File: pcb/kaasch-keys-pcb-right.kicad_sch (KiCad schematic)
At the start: 79 parts, among them SW1 SW_Push, SW10 SW_Push, SW11 SW_Push, SW12 SW_Push, SW13 SW_Push, SW14 SW_Push, SW15 SW_Push, SW16 SW_Push, SW17 SW_Push, SW18 SW_Push, SW19 SW_Push, SW2 SW_Push, SW20 SW_Push, SW21 SW_Push, SW22 SW_Push, SW23 SW_Push, SW24 SW_Push, SW25 SW_Push, SW26 SW_Push, SW27 SW_Push, SW28 SW_Push, SW29 SW_Push, SW3 SW_Push, SW30 SW_Push, SW31 SW_Push, SW32 SW_Push, SW33 SW_Push, SW34 SW_Push, SW35 SW_Push, SW36 SW_Push_Reset, SW4 SW_Push, SW5 SW_Push, SW6 SW_Push, SW7 SW_Push, SW8 SW_Push, SW9 SW_Push

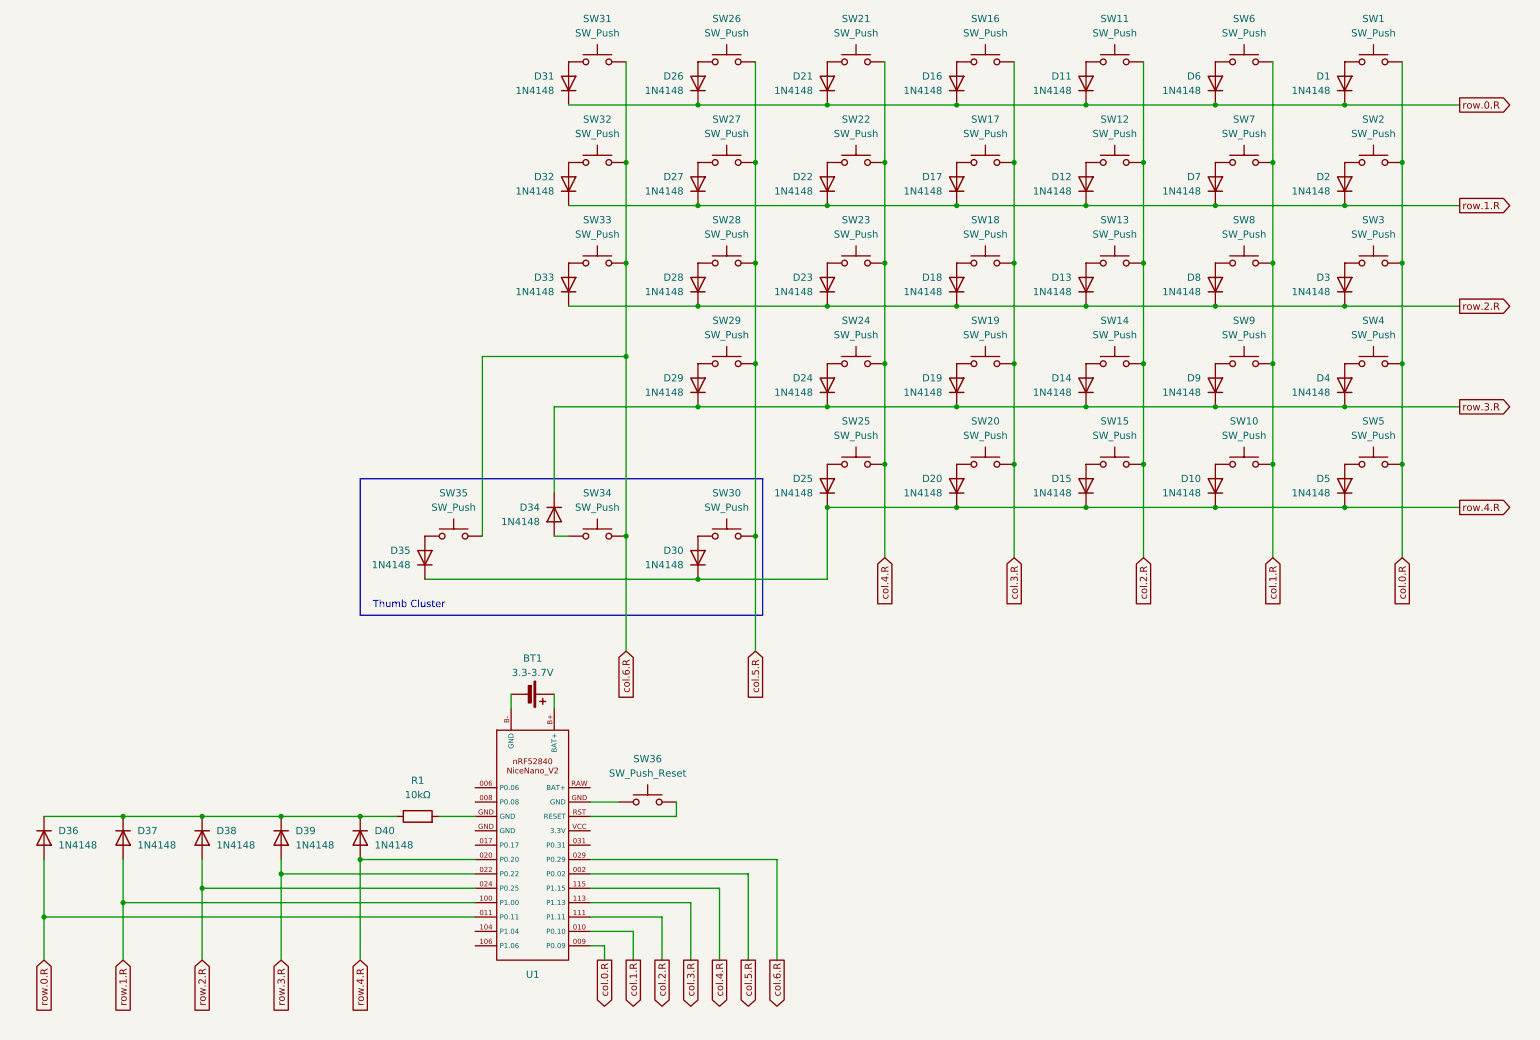
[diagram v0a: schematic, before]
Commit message: new naming and shit, big steps on left pcb
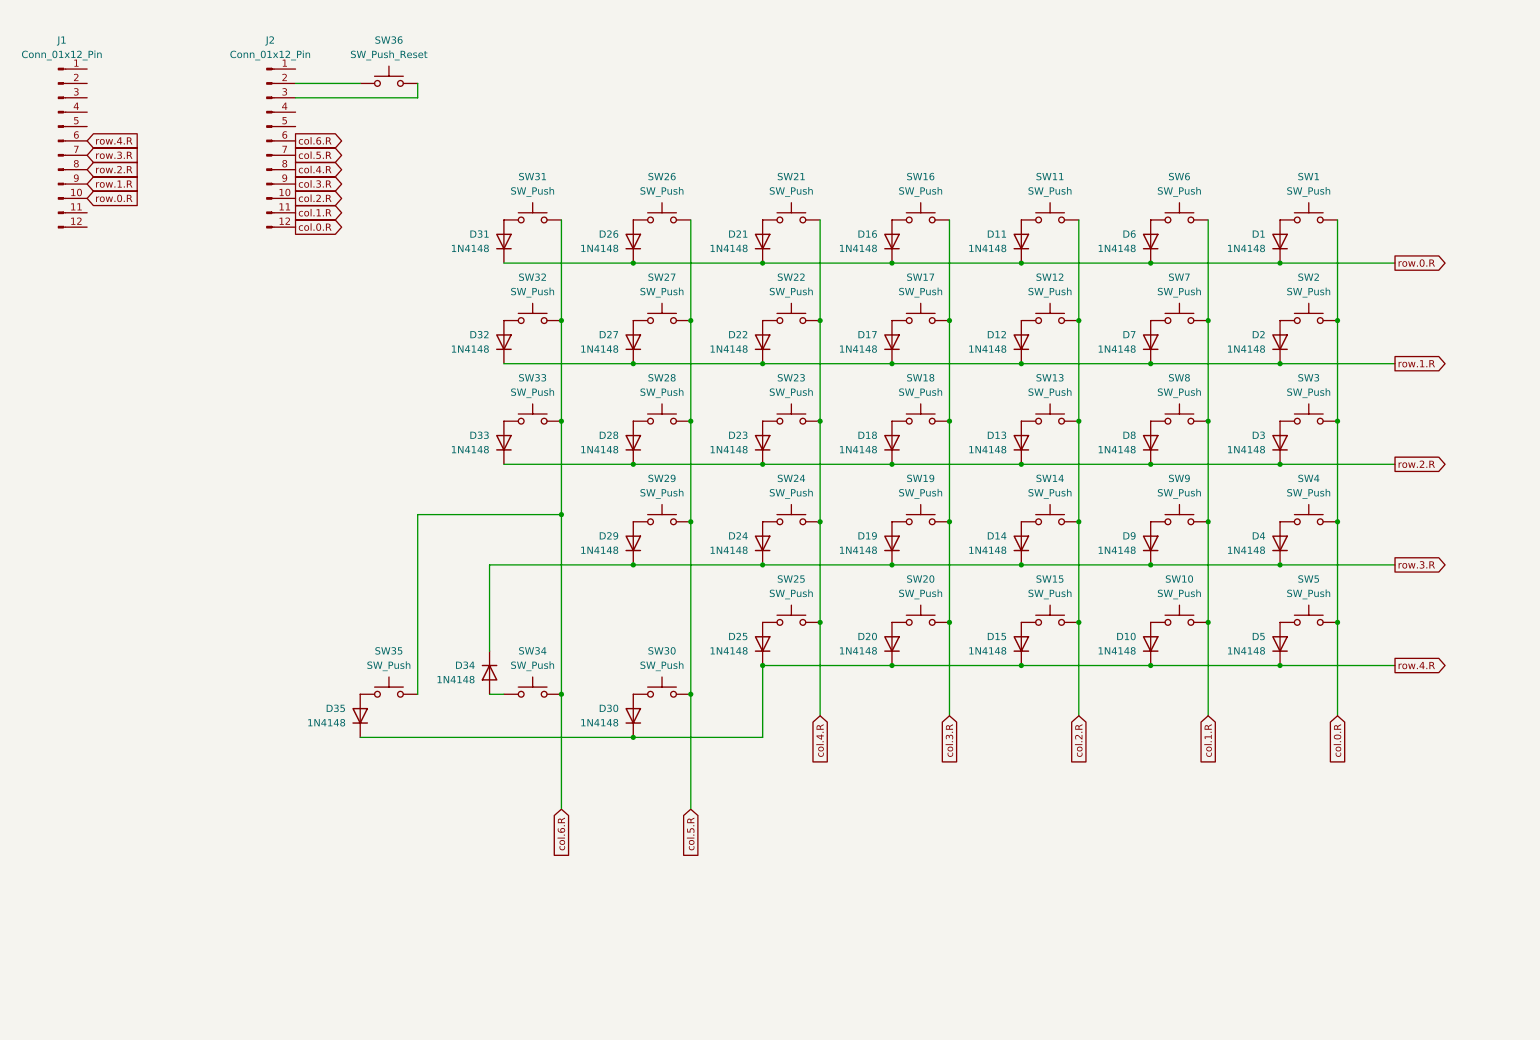
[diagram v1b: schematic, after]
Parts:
- removed BT1: 3.3-3.7V, symbol Device:Battery_Cell
- removed D36, D37, D38, D39, D40: 1N4148, Diode_SMD:D_1206_3216Metric, symbol Diode:1N4148
- removed R1: 10kΩ, Resistor_SMD:R_1206_3216Metric, symbol Device:R
- removed U1: ~, symbol NiceNanoV2:NiceNanoV2
- added J1, J2: Conn_01x12_Pin, symbol Connector:Conn_01x12_Pin
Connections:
- net col.0.R: now also J2.12 (Pin_12)
- net col.1.R: now also J2.11 (Pin_11)
- net col.2.R: now also J2.10 (Pin_10)
- net col.3.R: now also J2.9 (Pin_9)
- net col.4.R: now also J2.8 (Pin_8)
- net col.5.R: now also J2.7 (Pin_7)
- net col.6.R: now also J2.6 (Pin_6)
- net row.0.R: now also J1.10 (Pin_10)
- net row.1.R: now also J1.9 (Pin_9)
- net row.2.R: now also J1.8 (Pin_8)
- net row.3.R: now also J1.7 (Pin_7)
- net row.4.R: now also J1.6 (Pin_6)
- net at SW36.1: now also J2.2 (Pin_2)
- net at SW36.2: now also J2.3 (Pin_3)
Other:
- note removed: "Thumb Cluster"
- moved on the sheet: D1, D10, D11, D12, D13, D14, D15, D16, D17, D18, D19, D2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
